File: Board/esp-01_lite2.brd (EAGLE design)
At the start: 14 x 62 mm, 27 parts, among them IC1 TINY13-20SU

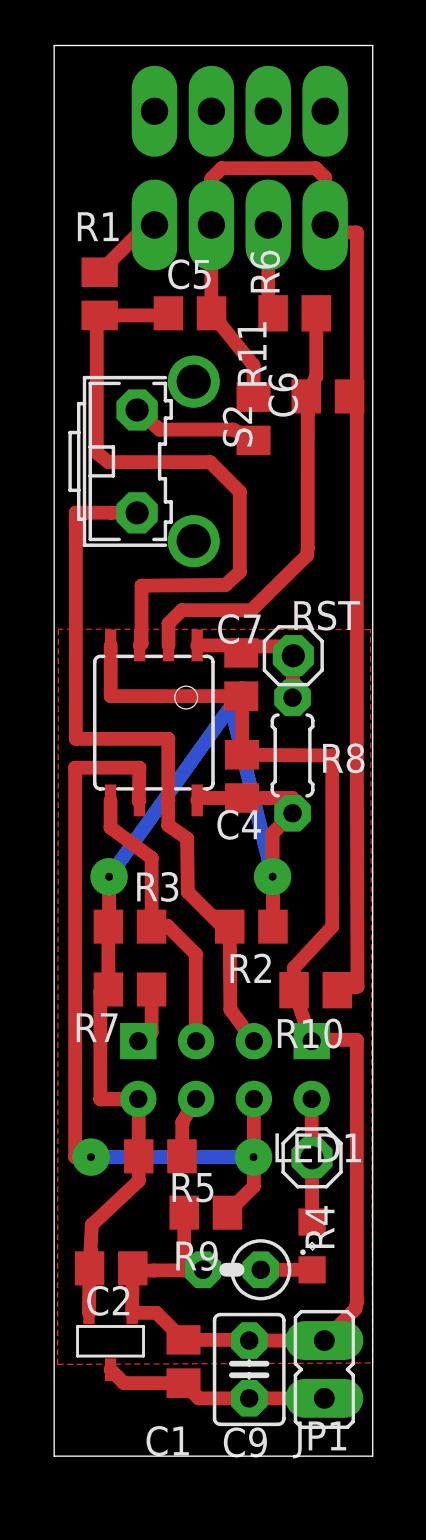
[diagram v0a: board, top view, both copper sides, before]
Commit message: board
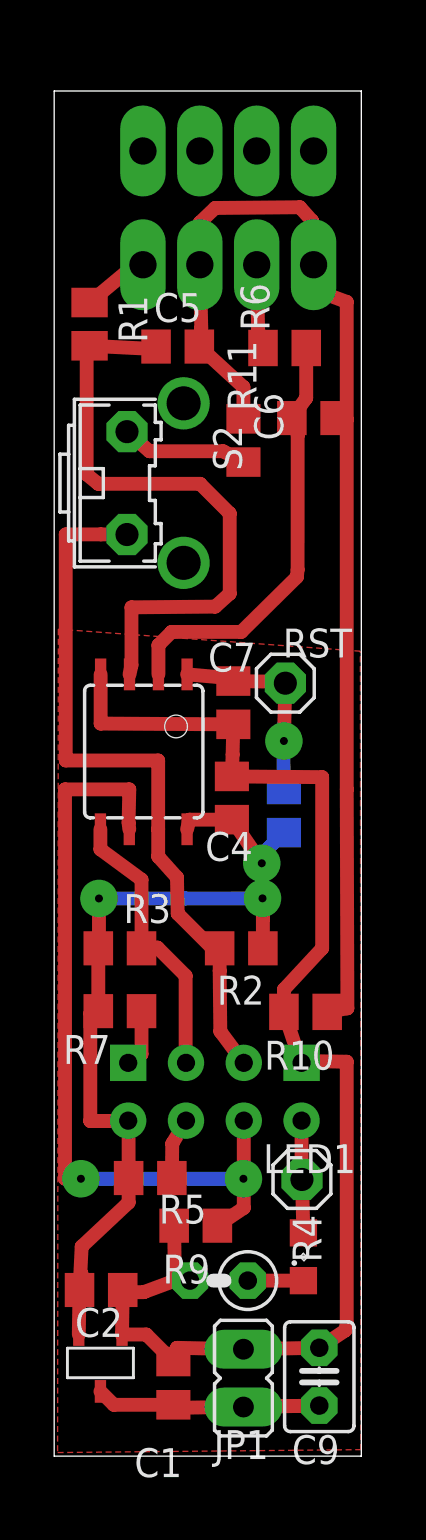
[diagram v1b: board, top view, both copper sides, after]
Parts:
- R11, R4: value 200 -> 300
- R8: device rcl:0204/5 -> rcl:R0805
- moved JP1 3.58 mm to (8.32, 3.43)
- moved C9 3.10 mm to (11.7, 3.49)
- moved R8 2.47 mm to (10.1, 28.4), flipped to the bottom
- moved X3 1.82 mm to (7.65, 54.9)
- moved R6 1.59 mm to (10.1, 48.7)
- moved C5 1.56 mm to (5.43, 48.8)
- moved R1 1.41 mm to (1.56, 49.8)
- moved IC1 1.35 mm to (3.94, 31.0)
- moved C7 1.29 mm to (7.87, 33.1)
- moved RST 1.26 mm to (10.2, 34.0)
- moved C6 1.14 mm to (11.4, 45.6)
- moved C4 1.05 mm to (7.81, 28.9)
- moved U$1 1.05 mm to (7.05, 22.9)
- moved C1 1.05 mm to (5.24, 3.21)
- moved R7 1.05 mm to (2.89, 19.6)
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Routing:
- net +3V3: track 51.7 -> 41.8 mm, vias 2 -> 3
- net AA*3: track 9.92 -> 13.2 mm
- net N$13: track 7.28 -> 10.3 mm, vias 0 -> 1
- net GND: track 61.1 -> 60.2 mm
- net GND1: track 54.1 -> 53.4 mm
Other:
- board size 14 x 62 mm -> 13.5 x 60 mm
